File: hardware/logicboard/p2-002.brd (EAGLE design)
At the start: 72 x 72 mm, 21 parts, among them IC1 74LS07N, U1 DS18B20

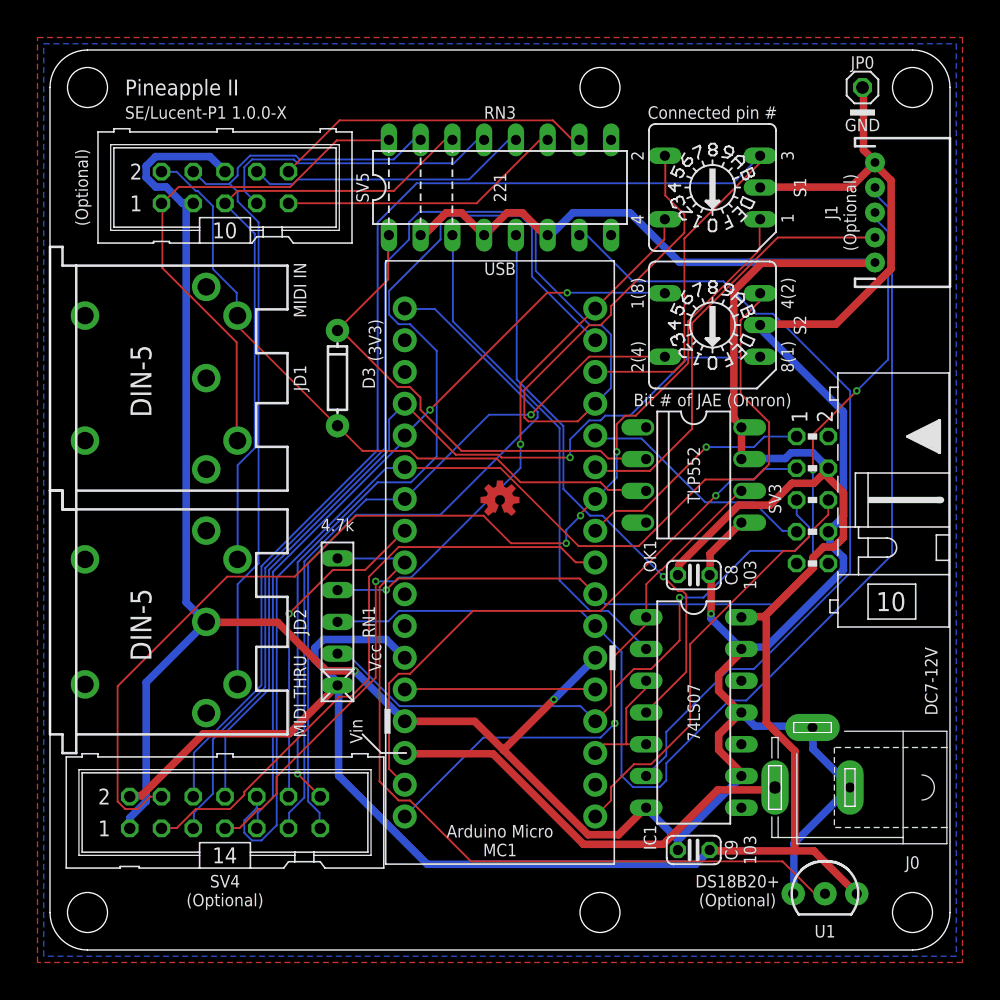
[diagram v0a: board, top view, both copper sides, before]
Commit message: Stepper Driver v0.0.2-X.
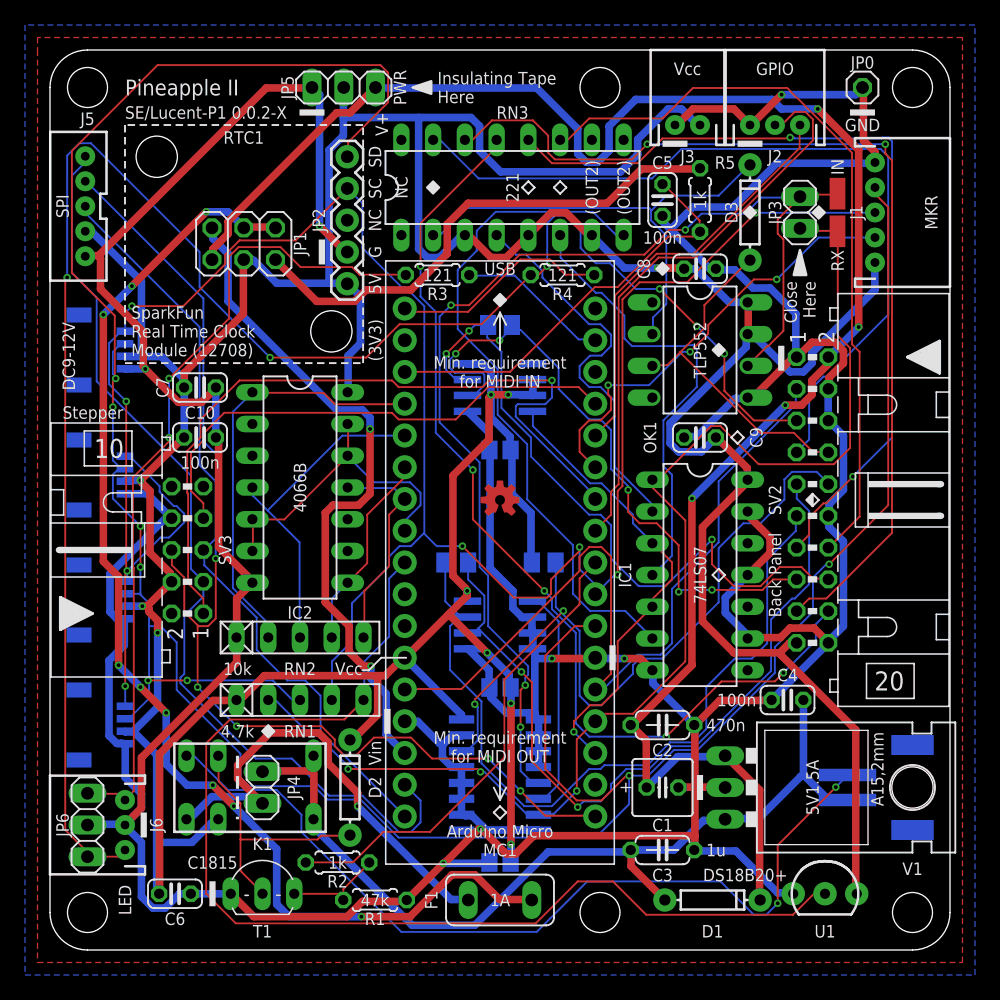
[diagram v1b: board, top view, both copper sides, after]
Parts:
- removed J0: (no value), con-jack:SPC4077
- removed JD1, JD2: DIN5, SparkFun-Connectors:DIN5-RA-PTH
- removed S1, S2: (no value), switch-dil:A1353HEX
- removed SV4: (no value), con-ml:ML14
- removed SV5: (no value), con-ml:ML10
- added C1: 22u, rcl:C025-050X050
- added C10, C4, C5: 100n, rcl:C025-024X044
- added C11, C12, C13: 10n, rcl:C2012
- added C2: 470n, rcl:C050-024X044
- added C3: 1u, rcl:C050-024X044
- added C6, C7: 10n, resistor:C025-024X044
- added D1, D2: (no value), SparkFun-DiscreteSemi:DIODE-1N4148
- added F1: 1.8A, fuse:TE5
- added H1, H2: STAND-OFF, SparkFun-Hardware:STAND-OFF
- added IC11: 74LS153D, 74xx-us:SO16
- added IC12, IC13: LTC485S, linear-technology:SOIC8
- added IC2: 4066N, 40xx:DIL14
- added IN, RX: (no value), wirepad:SMD1,27-2,54
- added J11, J12, J13, J14: Qwiic, SparkFun-Connectors:1X04_1MM_RA
- added J2: GPIO, SparkFun-Connectors:JST-3-PTH
- added J3: Vcc, SparkFun-Connectors:JST-2-PTH
- added J4: RLY, SparkFun-Connectors:JST-2-SMD
- added J5: SPI, SparkFun-Connectors:JST-5-PTH-VERT
- added J6: LED, SparkFun-Connectors:JST-3-PTH
- added JP1: PWRSEL, pinhead:2X03
- added JP2: RTC, SparkFun-Connectors:1X05
- added JP3: MPXJMP, pinhead:1X02
- added JP4: RLYJMP, pinhead:1X02
- added JP5: D5V, pinhead:1X03
- added JP6: LED, pinhead:1X03
- added K1: G5V1, relay:G5V1
- added R1: 47k, resistor:0204/5
- added R11: 10k, rcl:M2012
- added R12, R13: 120, rcl:M2012
- added R2, R5: 1k, resistor:0204/5
- added R3, R4: 120, resistor:0204/5
- added RN2: 10k, resistor-net:RN-5
- added SV2: (no value), con-ml:ML20L
- added T1: 2SC1815, transistor:TO92-ECB
- added V1: 5V, v-reg:78XXL
- J1: value (none) -> MKR
- RN3: value (none) -> 220
- moved SV3 50.2 mm to (11.0, 32.0), turned to 90 degrees
- moved D3 35.6 mm to (56.0, 59.0)
- moved C9 33.0 mm to (52.0, 41.0)
- moved C8 24.5 mm to (52.0, 54.5)
- moved IC1 11.0 mm to (52.0, 30.0)
- moved OK1 10.0 mm to (52.0, 48.0)
- moved RN1 6.93 mm to (20.0, 20.0), turned to 0 degrees
- moved RN3 1.00 mm to (37.0, 61.0)
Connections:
- new net ANLG1R: IC2.2
- new net ANLG2R: IC2.3
- new net ANLG3R: IC2.9
- new net ANLG4R: IC2.10
- new net LED0A: J6.1, JP6.1, R4.1, SV2.5
- new net LED1A: J6.3, JP6.3, R3.1
- new net MIN: IC11.5, IN.1, JP3.2, OK1.6
- new net MRX: IC11.6, IC12.1
- new net MRX+: IC12.6, R12.1, SV2.9
- new net MRX-: IC12.7, R12.2, SV2.11
- new net MRXDTCT: IC11.14, R11.1, SV2.10
- new net MTX+: IC13.6, R13.1, SV2.15
- new net MTX-: IC13.7, R13.2, SV2.16
- new net NC1: SV3.2
- new net NC2: SV3.9
- new net NC3: SV3.10
- new net RLYDRV: R1.2, R2.1, T1.B
- new net RLYOUT: J4.2, K1.10
- new net RLYSNK: D2.A, K1.9, T1.C
- new net V+: C1.1, C2.1, D1.C, JP1.1, JP5.3, SV2.2, V1.IN
- new net VCC/2: JP1.5, R5.2
- new net VOUT: F1.2, JP1.4, JP1.6
- new net VOUTRAW: C3.1, C4.1, D1.A, J4.1, JP4.2, K1.5, K1.6, V1.OUT
- new net VOUTRAW2: F1.1, JP4.1, K1.1
- net ANLG1: now also IC2.1, RN2.2; no longer S2.1, SV4.8
- net ANLG2: now also IC2.4, RN2.3; no longer S2.2, SV4.9
- net ANLG3: now also IC2.8, RN2.4; no longer S2.4, SV4.10
- net ANLG4: now also IC2.11, RN2.5; no longer S2.8, SV4.11
- net AREF: now also C5.1, R5.1
- net DTCT1: now also SV3.1; no longer S1.1, SV4.4
- net DTCT2: now also SV3.7; no longer S1.2, SV4.5
- net DTCT3: no longer S1.4, SV4.6
- net DTCT4: no longer S1.8, SV4.7
- net GATE: now also IC2.12, IC2.13, IC2.5, IC2.6; no longer SV4.12
- net GND: now also C1.2, C10.2, C11.2, C12.2, C13.2, C2.2, C3.2, C4.2, C5.2, C6.2, C7.2, IC11.1, IC11.10, IC11.11, IC11.12, IC11.13, IC11.15, IC11.2, IC11.3, IC11.4, IC11.8, IC12.2, IC12.3, IC12.4, IC12.5, IC13.5, IC2.7, J11.1, J12.1, J13.1, J14.1, J2.1, J3.1, J5.1, J6.2, JP2.2, JP5.1, JP6.2, R1.1, RN2.1, SV2.1, SV2.12, SV2.20, SV2.4, SV2.6, T1.E, V1.GND; no longer J0.1, J0.2, JD2.2, S1.C, S2.C, SV4.1, SV5.3, SV5.6
- net GPIO1: now also J2.2; no longer SV3.1
- net GPIO2: now also J2.3; no longer SV3.7
- net LED0: now also R4.2; no longer SV4.13
- net LED1: now also R3.2; no longer SV4.14
- net MIDIINSND: now also RN3.2; no longer RN3.1
- net MIRTN: now also SV2.8; no longer JD1.5, SV5.2
- net MISND: now also RN3.15, SV2.7; no longer JD1.4, RN3.16, SV5.1
- net MISO: now also J5.5
- net MO: now also RN3.6; no longer RN3.5
- net MO2: now also RN3.8; no longer RN3.7
- net MO2RTN: now also RN3.9; no longer RN3.10, SV5.10
- net MO2SND: now also RN3.10; no longer RN3.11, SV5.9
- net MORTN: now also RN3.11, SV2.14; no longer RN3.12, SV5.8
- net MOSI: now also J5.4
- net MOSND: now also RN3.12, SV2.13; no longer RN3.13, SV5.7
- net MT: now also RN3.4; no longer RN3.3
- net MTRTN: now also RN3.13, SV2.18; no longer JD2.5, RN3.14, SV5.5
- net MTSND: now also RN3.14, SV2.17; no longer JD2.4, RN3.15, SV5.4
- net RLY: now also R2.2; no longer SV4.3
- net RST: now also SV2.3
- net RX: now also IC11.7, JP3.1, RX.1; no longer OK1.6
- net SCK: now also J5.3
- net SCL: now also J11.4, J12.4, J13.4, J14.4, JP2.4
- net SDA: now also J11.3, J12.3, J13.3, J14.3, JP2.5
- net TX: now also IC13.4
- net VCC: now also C10.1, C11.1, C12.1, C13.1, C6.1, C7.1, D2.C, IC11.16, IC12.8, IC13.2, IC13.3, IC13.8, IC2.14, J11.2, J12.2, J13.2, J14.2, J3.2, J5.2, JP1.3, JP2.1, JP5.2, K1.2, R11.2, RN3.3, RN3.5, RN3.7, SV2.19; no longer RN3.2, RN3.4, RN3.6, SV4.2
- net VIN: now also JP1.2; no longer J0.3
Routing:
- net VCC: track 214.3 -> 399.5 mm, vias 0 -> 10
- net GND: track 251.4 -> 430.2 mm, vias 3 -> 7
- net V+: track 0.00 -> 147.0 mm, vias 0 -> 4
- net LED0A: track 0.00 -> 143.7 mm, vias 0 -> 6
- net SDA: track 94.8 -> 237.7 mm, vias 0 -> 8
- net SCL: track 71.7 -> 186.6 mm, vias 3 -> 8
- net DTCT3: track 111.3 -> 0.00 mm
- net VOUT: track 0.00 -> 94.9 mm, vias 0 -> 9
- net MIN: track 0.00 -> 93.0 mm, vias 0 -> 4
- net DTCT2: track 118.2 -> 41.5 mm
- net ANLG3: track 90.1 -> 16.0 mm
- net VOUTRAW: track 0.00 -> 73.7 mm
- net RLYOUT: track 0.00 -> 69.7 mm, vias 0 -> 2
- net DTCT4: track 65.6 -> 0.00 mm, vias 2 -> 0
- net LED1A: track 0.00 -> 65.6 mm, vias 0 -> 2
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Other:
- board text added: "(OUT2)"
- board text added: "+"
- board text added: "100n"
- board text added: "10k"
- board text added: "121"
- board text added: "1A"
- board text added: "1k"
- board text added: "1u"
- board text added: "4066B"
- board text added: "470n"
- board text added: "47k"
- board text added: "5V"
- board text added: "5V1.5A"
- board text added: "74153"
- board text added: "Arduino"
- board text added: "Back Panel"
- board text added: "Bottom View"
- board text added: "C1815"
- board text added: "Close"
- board text added: "Close Here"
- board text added: "D7"
- board text added: "DC9-12V"
- board text added: "Direct 5V"
- board text added: "Don't Close"
- board text added: "Dual"
- board text added: "Ext. V+"
- board text added: "G"
- board text added: "G1"
- board text added: "G2"
- board text added: "GPIO"
- board text added: "IN-RX"
- board text added: "Insulating Tape Here"
- board text added: "LED"
- board text added: "LED0"
- board text added: "LED1"
- board text added: "LTC485"
- board text added: "MI"
- board text added: "MKR"
- board text added: "MO"
- board text added: "Min. requirement for MIDI IN"
- board text added: "Min. requirement for MIDI OUT"
- board text added: "NC"
- board text added: "OUT"
- board text added: "Open JP1"
- board text added: "PWR"
- board text added: "PWRSEL"
- board text added: "Qwiic/5V"
- board text added: "RLYJMP"
- board text added: "RTC1"
- board text added: "RTN"
- board text added: "RX"
- board text added: "Regulator"
- board text added: "Relay"
- board text added: "SC"
- board text added: "SCK"
- board text added: "SCL"
- board text added: "SD"
- board text added: "SDA"
- board text added: "SE/Lucent-P1 0.0.2-X"
- board text added: "SND"
- board text added: "SPI"
- board text added: "SparkFun Real Time Clock Module (12708)"
- board text added: "Stepper"
- board text added: "TX"
- board text added: "V+"
- board text added: "Vcc/2"
- board text added: "Vin (MC)"
- board text added: "Vout"
- board text added: "Vout (Reg)"
- board text added: "Voutraw"
- board text removed: "(Optional)"
- board text removed: "1"
- board text removed: "1(8)"
- board text removed: "103"
- board text removed: "2"
- board text removed: "2(4)"
- board text removed: "3"
- board text removed: "4"
- board text removed: "4(2)"
- board text removed: "8(1)"
- board text removed: "Bit # of JAE (Omron)"
- board text removed: "Connected pin #"
- board text removed: "DC7-12V"
- board text removed: "MIDI IN"
- board text removed: "MIDI THRU"
- board text removed: "SE/Lucent-P1 1.0.0-X"
- board text removed: "STEPPER"
